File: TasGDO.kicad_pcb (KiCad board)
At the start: 2 copper layers, 46 x 44 mm, 37 parts, among them J2 Conn_01x04_Pin, J3 Screw_Terminal_01x02, J4 Screw_Terminal_01x02, J6 Screw_Terminal_01x03, K1 AQY212GSX, SW1 SW_Push, SW2 SW_Push, U1 ESP32-S3-MINI-2, U2 TPS56339DDCR

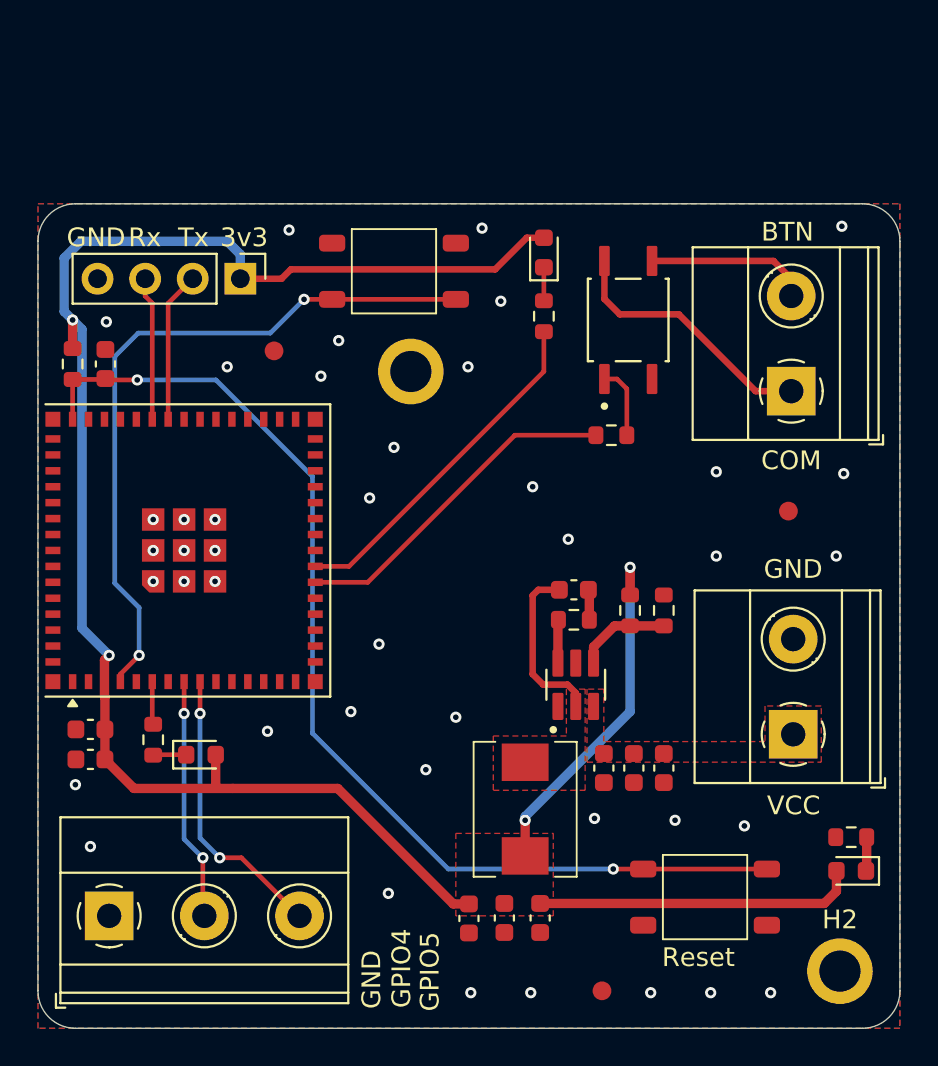
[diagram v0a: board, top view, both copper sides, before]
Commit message: feat: miniturise the board
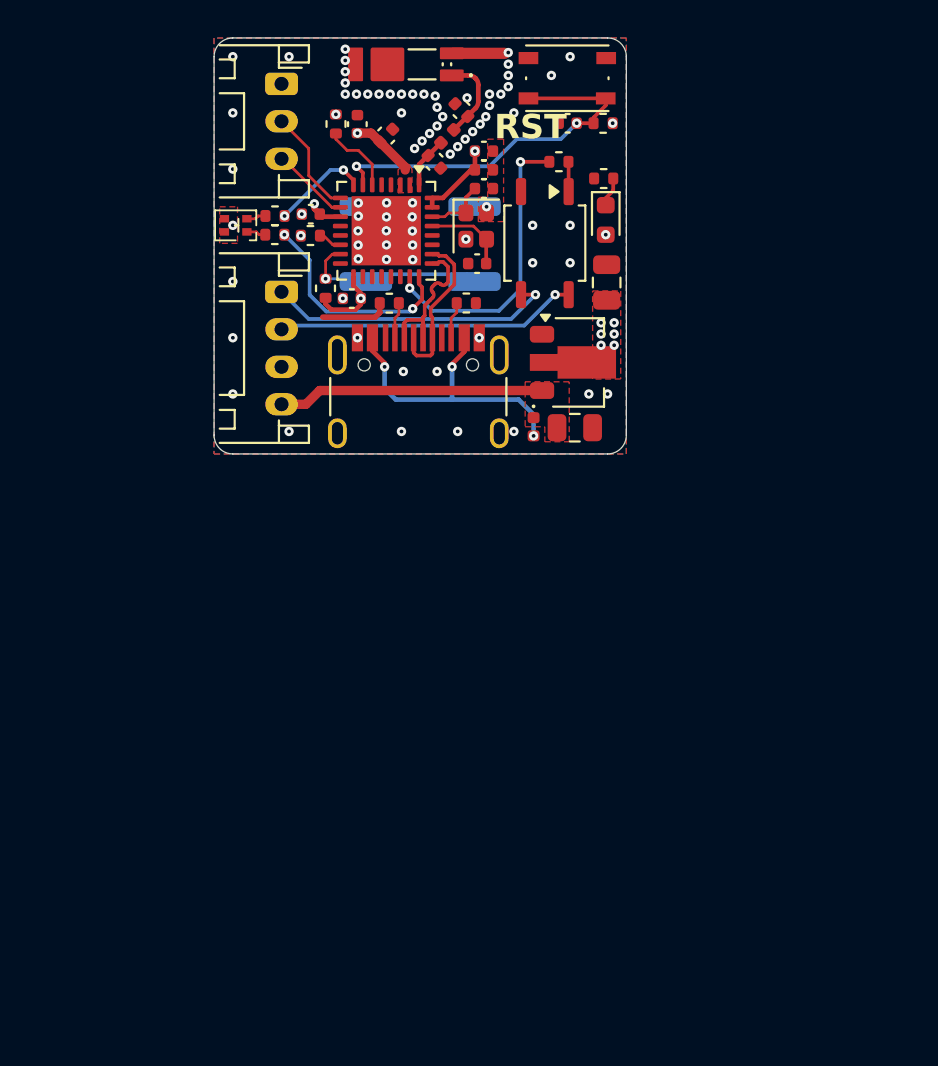
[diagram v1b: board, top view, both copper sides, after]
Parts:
- removed C10, C8: 22u, Capacitor_SMD:C_0603_1608Metric
- removed C5: 10u, Capacitor_SMD:C_0603_1608Metric
- removed C7: 100n, Capacitor_SMD:C_0603_1608Metric
- removed D2: B, LED_SMD:LED_0603_1608Metric
- removed D3: Red, LED_SMD:LED_0603_1608Metric
- removed FID1, FID2, FID3: Fiducial, Fiducial:Fiducial_1mm_Mask2mm
- removed G***: LOGO, tasgdo:Logo
- removed H1, H2: MountingHole, MountingHole:MountingHole_2.2mm_M2_ISO7380_Pad
- removed J2: Conn_01x04_Pin, Connector_PinHeader_2.54mm:PinHeader_1x04_P2.54mm_Vertical
- removed J4: Screw_Terminal_01x02, TerminalBlock_Phoenix:TerminalBlock_Phoenix_MKDS-1,5-2-5.08_1x02_P5.08mm_Horizontal
- removed J6: Screw_Terminal_01x03, TerminalBlock_Phoenix:TerminalBlock_Phoenix_MKDS-1,5-3-5.08_1x03_P5.08mm_Horizontal
- removed R9: 10K, Resistor_SMD:R_0603_1608Metric
- removed U1: ESP32-S3-MINI-2, tasgdo:ESP32-S2-MINI-1
- added AE1: Ant_RFECA3216060A1T_1206, Hardware Components:Ant_RFECA3216060A1T, F.Cu at (144.4, 61.5)
- added C23: 12pF, Hardware Components:C_0402_1005Metric, F.Cu at (147.8, 68.2)
- added C24: 12pF, Hardware Components:C_0402_1005Metric, F.Cu at (147.4, 72.2)
- added C25: 2p7, Hardware Components:C_0402_1005Metric, F.Cu at (145.2, 66.8)
- added C26: 2p4, Hardware Components:C_0402_1005Metric, F.Cu at (146.6, 64.0)
- added C29: 100n, Hardware Components:C_0402_1005Metric, F.Cu at (138.6, 69.5)
- added C30: 100n, Hardware Components:C_0402_1005Metric, F.Cu at (140.8, 74.0)
- added C34: 1u, Hardware Components:C_0402_1005Metric, F.Cu at (147.8, 66.2)
- added D1: D_Schottky_Small, Hardware Components:D_0402_1005Metric, F.Cu at (150.4, 80.9)
- added D5: LED_Dual_AAKK, Hardware Components:LED_LiteOn_LTST-C295K_1.6x0.8mm, F.Cu at (134.6, 70.2)
- added J1: Conn_01x04, Hardware Components:Conn_JST_PH_S4B-PH-K_1x04_P2.00mm_Horizontal, F.Cu at (137.0, 73.7)
- added J10: USB_C_Receptacle_USB2.0_16P, Hardware Components:USB_C_Receptacle_HRO_TYPE-C-31-M-12, F.Cu at (144.3, 80.2)
- added R13: 5k1, Hardware Components:R_0402_1005Metric, F.Cu at (142.8, 74.3)
- added R14: 5k1, Hardware Components:R_0402_1005Metric, F.Cu at (146.9, 74.3)
- added R3: 10k, Hardware Components:R_0402_1005Metric, F.Cu at (139.9, 64.7)
- added U3: ESP32-C3, Hardware Components:QFN-32-1EP, F.Cu at (142.6, 70.4)
- added Y2: ECS-400-10-37B2-CKM-TR, Hardware Components:Oscillator_ECS_400-10-37B2-CKM-TR, F.Cu at (147.4, 70.2)
- C1, C3, C4: footprint Capacitor_SMD:C_0603_1608Metric -> Hardware Components:C_0402_1005Metric
- C2: value 100n -> 10n; footprint Capacitor_SMD:C_0603_1608Metric -> Hardware Components:C_0402_1005Metric
- C6: footprint Capacitor_SMD:C_0603_1608Metric -> Hardware Components:C_0805_2012Metric
- C9: value 100n -> 10u; footprint Capacitor_SMD:C_0603_1608Metric -> Hardware Components:C_0805_2012Metric
- D4: footprint LED_SMD:LED_0603_1608Metric -> Hardware Components:LED_0603_1608Metric
- J3: value Screw_Terminal_01x02 -> Conn_01x03; footprint TerminalBlock_Phoenix:TerminalBlock_Phoenix_MKDS-1,5-2-5.08_1x02_P5.08mm_Horizontal -> Hardware Components:Conn_JST_PH_S3B-PH-K_1x03_P2.00mm_Horizontal
- K1: footprint tasgdo:SOIC254P680X230-4N -> Hardware Components:SSR_SUPSiC_GAQY212GSX
- L1: value 4.7uH -> 2.4nH; footprint tasgdo:YSPI0530 -> Hardware Components:L_0402_1005Metric
- R1, R2, R4, R5, R6: footprint Resistor_SMD:R_0603_1608Metric -> Hardware Components:R_0402_1005Metric
- R7: value 30 -> 10k; footprint Resistor_SMD:R_0603_1608Metric -> Hardware Components:R_0402_1005Metric
- R8: value 30.9K -> 10k; footprint Resistor_SMD:R_0603_1608Metric -> Hardware Components:R_0402_1005Metric
- SW1: footprint tasgdo:K2-1109SP-B4SA-01 -> Hardware Components:SW_PTS815SJM250SMTRLFS
- SW2: value SW_Push -> KSC241J LFS; footprint tasgdo:K2-1109SP-B4SA-01 -> Hardware Components:SW_CK_KSC241JLFS; moved to B.Cu
- U2: value TPS56339DDCR -> Conv_AMS1117S-3.3; footprint tasgdo:TPS56339DDCR -> Hardware Components:SOT-89-3
- moved SW1 44.3 mm to (152.2, 62.3), turned to 0 degrees
- moved R6 37.6 mm to (154.2, 67.7)
- moved D4 37.1 mm to (154.3, 69.9), turned to -90 degrees
- moved C4 36.8 mm to (141.1, 64.8), turned to 90 degrees
- moved L1 36.2 mm to (145.8, 65.4), turned to 45 degrees
- moved C3 35.4 mm to (142.6, 65.4), turned to 45 degrees
- moved C9 34.1 mm to (154.3, 73.2), turned to -90 degrees
- moved J3 31.8 mm to (137.0, 62.6), turned to -90 degrees
- moved R1 31.1 mm to (154.2, 64.7), turned to 180 degrees
- moved R4 28.7 mm to (136.7, 69.7), turned to 0 degrees
- moved C1 27.8 mm to (152.3, 64.7), turned to 180 degrees
- moved R7 24.9 mm to (138.5, 70.7)
- moved R8 23.7 mm to (139.3, 73.5)
- moved C2 22.9 mm to (147.8, 67.2), turned to 0 degrees
- moved C6 18.8 mm to (152.7, 81.0), turned to 180 degrees
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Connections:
- net Net-(J4-Pin_1) renamed VCC
- C2 pad 1: Net-(C2-Pad1) -> +3.3V
- C2 pad 2: Net-(U2-SW) -> GND
- J3 pad 1: Net-(J3-Pin_1) -> GND
- J3 pad 2: Net-(J3-Pin_2) -> /GPIO4
- K1 pad 3: Net-(J3-Pin_2) -> /COM
- K1 pad 4: Net-(J3-Pin_1) -> /BTN
- L1 pad 1: Net-(U2-SW) -> /RF_ANT
- L1 pad 2: +3.3V -> /RF_FEED
- R7 pad 1: Net-(U2-BOOT) -> +3.3V
- R7 pad 2: Net-(C2-Pad1) -> Net-(U3-GPIO8)
- R8 pad 1: Net-(U2-FB) -> +3.3V
- R8 pad 2: +3.3V -> /BOOT_OPT
- U2 pad 2: Net-(U2-SW) -> +3.3V
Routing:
- net +3.3V: track 118.6 -> 13.8 mm, vias 4 -> 14
- net /EN: track 58.1 -> 20.5 mm
- net /BOOT_OPT: track 37.8 -> 10.7 mm, vias 2 -> 1
- net /VBUS: track 0.00 -> 16.2 mm, vias 0 -> 3
- net /BTN: track 0.00 -> 16.1 mm, vias 0 -> 1
- net /COM: track 0.00 -> 15.5 mm, vias 0 -> 1
- net VCC: track 0.00 -> 14.2 mm
- net Net-(J3-Pin_1): track 14.0 -> 0.00 mm
- net /GPIO5: track 15.4 -> 4.21 mm, vias 2 -> 0
- net Net-(U2-SW): track 9.19 -> 0.00 mm
- net Net-(J3-Pin_2): track 8.74 -> 0.00 mm
- net /USB_P: track 0.00 -> 8.63 mm
- net /USB_N: track 0.00 -> 8.59 mm
- net /TX: track 8.04 -> 0.00 mm
- net /RX: track 7.66 -> 0.00 mm
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- added copper zone on In2.Cu, net +3.3V
- added copper zone on In1.Cu, net GND
- removed copper zone on F.Cu, net Net-(U2-SW)
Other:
- board size 46 x 44 mm -> 22 x 22.2 mm
- copper layers 2 -> 4
- board text added: "0"
- board text added: "0 mm"
- board text added: "0.01 mm"
- board text added: "0.0152 mm"
- board text added: "0.02"
- board text added: "0.035 mm"
- board text added: "0.127 mm / 0.15 mm"
- board text added: "0.2000 mm"
- board text added: "0.2104 mm"
- board text added: "1"
- board text added: "1.065 mm"
- board text added: "1.6062 mm"
- board text added: "22 mm x 22 mm"
- board text added: "3.3"
- board text added: "4"
- board text added: "4.4"
- board text added: "4.6"
- board text added: "7628"
- board text added: "B.Cu"
- board text added: "B.Mask"
- board text added: "B.Paste"
- board text added: "B.Silkscreen"
- board text added: "BOARD CHARACTERISTICS"
- board text added: "Black"
- board text added: "Board Thickness:"
- board text added: "Board overall dimensions:"
- board text added: "Bottom Silk Screen"
- board text added: "Bottom Solder Mask"
- board text added: "Bottom Solder Paste"
- board text added: "Castellated pads:"
- board text added: "Color"
- board text added: "Copper Finish:"
- board text added: "Copper Layer Count:"
- board text added: "Dielectric 1"
- board text added: "Dielectric 2"
- board text added: "Dielectric 3"
- board text added: "Edge card connectors:"
- board text added: "Epsilon R"
- board text added: "F.Cu"
- board text added: "F.Mask"
- board text added: "F.Paste"
- board text added: "F.Silkscreen"
- board text added: "FR4"
- board text added: "HASL"
- board text added: "Impedance Control:"
- board text added: "Impedance control"
- board text added: "In1.Cu"
- board text added: "In2.Cu"
- board text added: "Layer Name"
- board text added: "Loss Tangent"
- board text added: "Material"
- board text added: "Min hole diameter:"
- board text added: "Min track/spacing:"
- board text added: "No"
- board text added: "Plated Board Edge:"
- board text added: "RST"
- board text added: "Thickness (mm)"
- board text added: "Top Silk Screen"
- board text added: "Top Solder Mask"
- board text added: "Top Solder Paste"
- board text added: "Type"
- board text added: "White"
- board text added: "Yes"
- board text added: "copper"
- board text added: "core"
- board text added: "prepreg"
- board text added: "v0.3"
- board text removed: "3v3"
- board text removed: "BTN"
- board text removed: "COM"
- board text removed: "GND"
- board text removed: "GPIO4"
- board text removed: "GPIO5"
- board text removed: "Reset"
- board text removed: "Rx"
- board text removed: "Tx"
- board text removed: "VCC"
- board text removed: "v0.2"

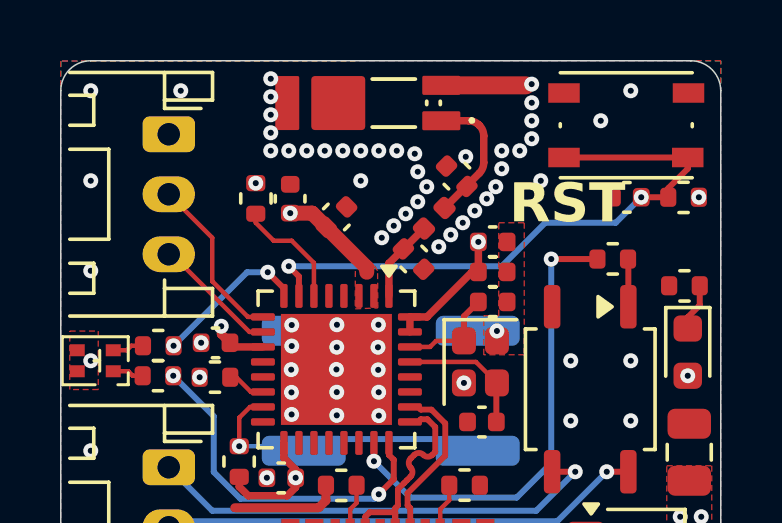
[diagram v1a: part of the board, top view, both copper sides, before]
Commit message: fix: 50 ohn trace
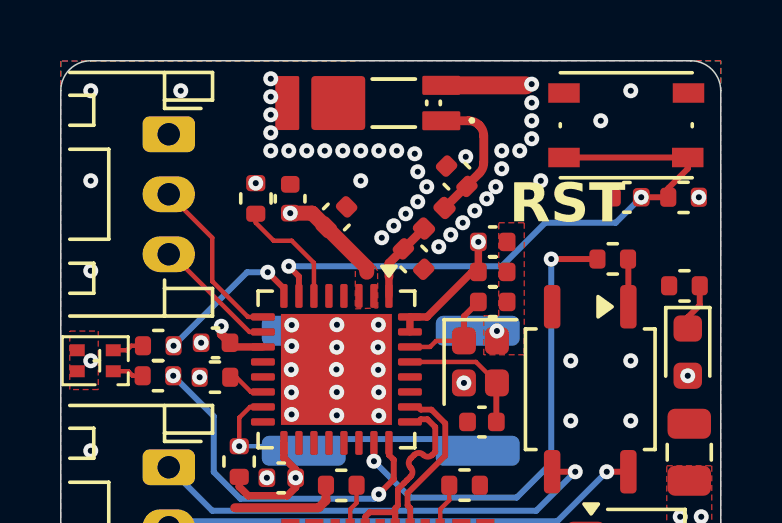
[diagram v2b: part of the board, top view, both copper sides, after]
